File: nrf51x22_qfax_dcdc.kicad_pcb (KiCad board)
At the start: 2 copper layers, 14.8 x 16.4 mm, 46 parts, among them U1 nrf51822-qfax, X1 Crystal-4, X2 32.768kHz

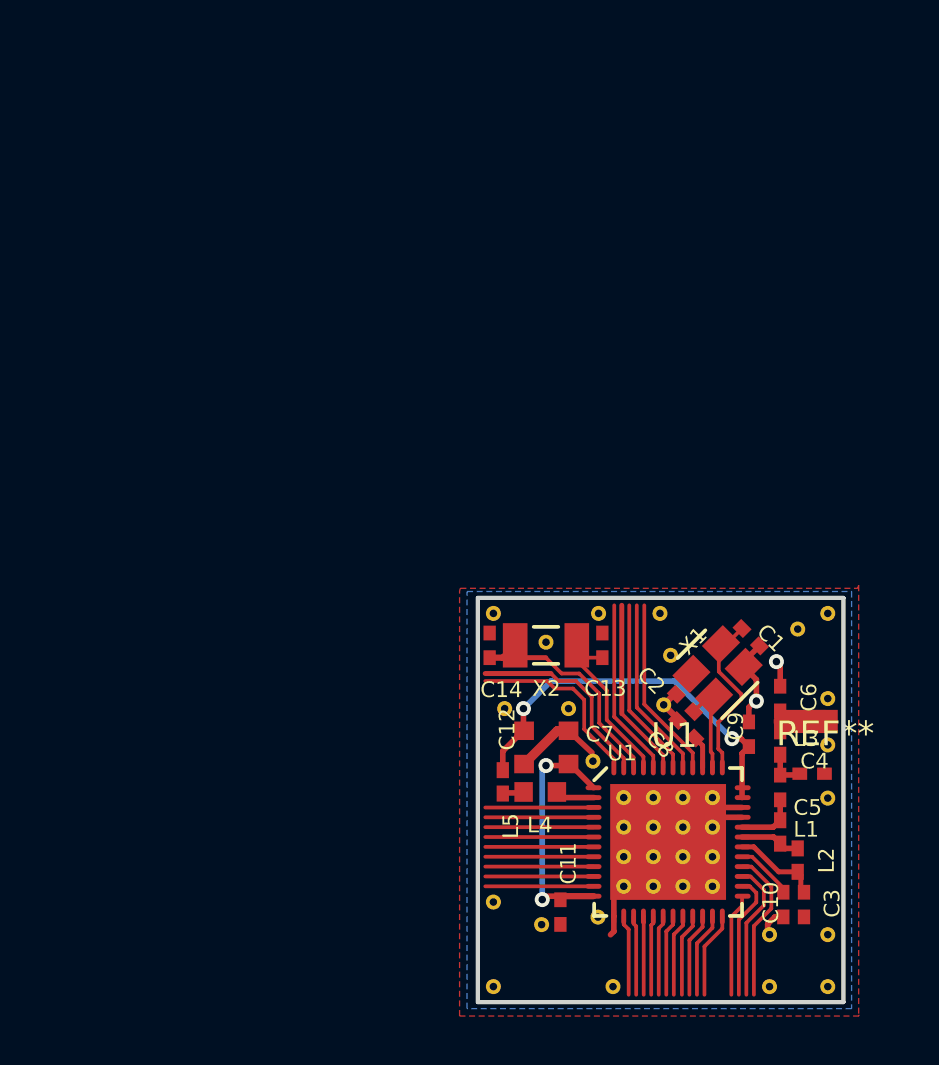
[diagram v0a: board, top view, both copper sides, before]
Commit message: WIP: Adding finished sch
Signed-off-by: Zamir SUN <sztsian@gmail.com>
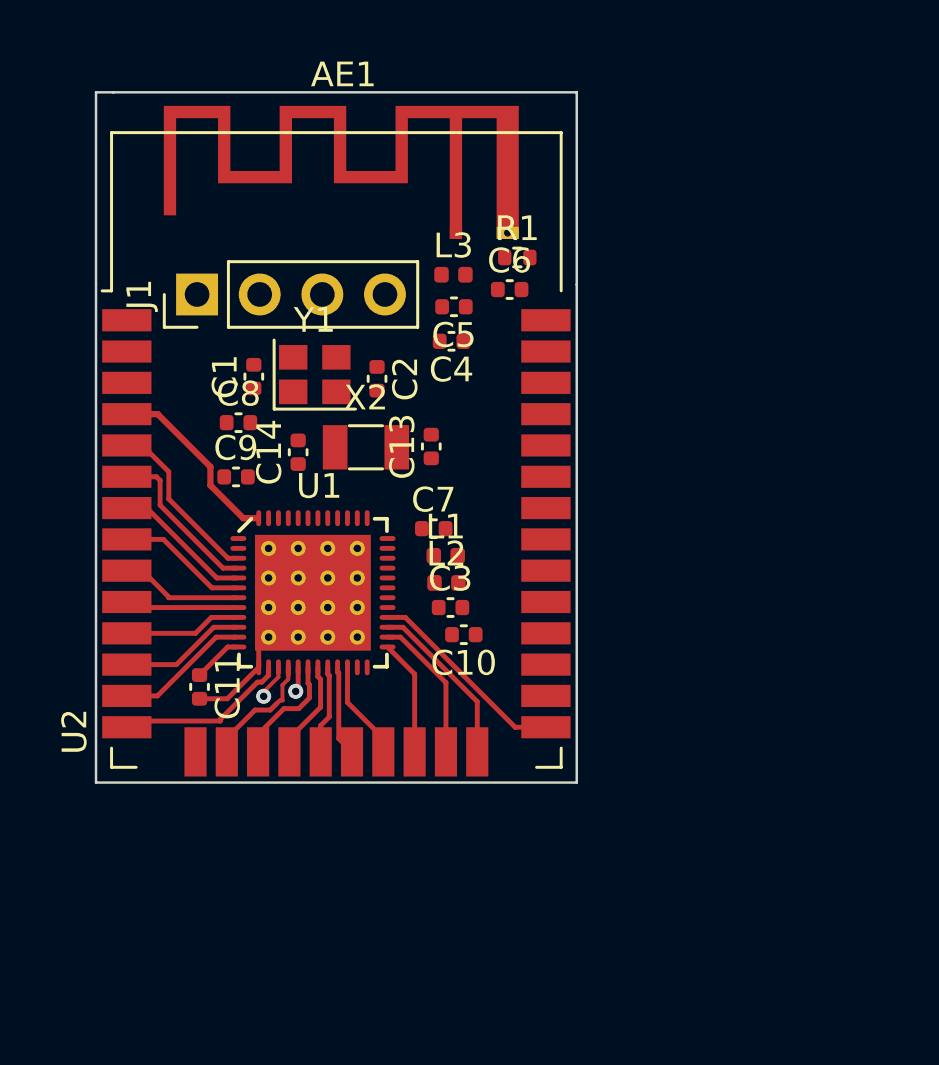
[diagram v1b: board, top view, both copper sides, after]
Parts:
- removed C12: 1.0uF, dcdc:CAPC1608X06L
- removed L4: 10uH, dcdc:INDC1608X06L
- removed L5: 15nH, dcdc:INDC1005X04L
- removed REF** (x23): VIA-0.6096, dcdc:VIA-0.6096
- removed REF**: antenna, dcdc:antenna
- removed X1: Crystal-4, dcdc:BT-XTAL_2520
- added AE1: Antenna_Chip, RF_Antenna:Texas_SWRA117D_2.4GHz_Left, F.Cu at (75.5, -110.2)
- added J1: SWD, Connector_PinHeader_2.54mm:PinHeader_1x04_P2.54mm_Vertical, F.Cu at (65.0, -107.7)
- added R1: 0R, Resistor_SMD:R_0402_1005Metric, F.Cu at (78.0, -109.2)
- added U2: nRF51822-WROOM-32, zsun-symbols:nRF51822-WROOM-32D, F.Cu at (70.7, -98.4)
- added Y1: 16M 3225, Crystal:Crystal_SMD_2520-4Pin_2.5x2.0mm, F.Cu at (69.8, -104.5)
- C1, C10, C11, C13, C14, C2, C3, C4, C5, C6, C8, C9: footprint dcdc:CAPC1005X04L -> Capacitor_SMD:C_0402_1005Metric
- C7: footprint dcdc:CAPC1608X06L -> Capacitor_SMD:C_0402_1005Metric
- L1, L2, L3: footprint dcdc:INDC1005X04L -> Inductor_SMD:L_0402_1005Metric
- X2: footprint dcdc:XTAL_3215 -> Crystal:Crystal_SMD_3215-2Pin_3.2x1.5mm
- moved C5 23.6 mm to (75.4, -107.2), turned to 180 degrees
- moved C9 23.3 mm to (66.6, -100.3), turned to 0 degrees
- moved L3 23.2 mm to (75.4, -108.5), turned to 0 degrees
- moved C4 22.8 mm to (75.3, -105.8), turned to 180 degrees
- moved C1 22.8 mm to (67.3, -104.4), turned to 90 degrees
- moved C8 22.0 mm to (66.7, -102.5), turned to 0 degrees
- moved C6 19.9 mm to (77.7, -107.9), turned to 0 degrees
- moved C3 18.7 mm to (75.3, -95.0), turned to 0 degrees
- moved L2 18.2 mm to (75.1, -96.0)
- moved C2 18.1 mm to (72.3, -104.3), turned to 270 degrees
- moved U1 17.6 mm to (69.7, -95.6)
- moved L1 17.6 mm to (75.1, -97.1)
- moved C11 17.3 mm to (65.1, -91.8)
- moved C10 17.0 mm to (75.8, -93.9), turned to 180 degrees
- moved C14 11.0 mm to (69.1, -101.3), turned to 90 degrees
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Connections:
- C11 pad 1: Net-(C11-Pad1) -> /AVDD
- C7 pad 1: Net-(C11-Pad1) -> /AVDD
- C9 pad 1: Net-(C12-Pad1) -> /AVDD
- U1 pad 1: Net-(C11-Pad1) -> /AVDD
- U1 pad 10: (no net) -> /P0.06
- U1 pad 11: (no net) -> /P0.07
- U1 pad 12: Net-(C11-Pad1) -> /AVDD
- U1 pad 14: (no net) -> /P0.08
- U1 pad 15: (no net) -> /P0.09
- U1 pad 16: (no net) -> /P0.10
- U1 pad 17: (no net) -> /P0.11
- U1 pad 18: (no net) -> /P0.12
- U1 pad 19: (no net) -> /P0.13
- U1 pad 2: Net-(L4-Pad2) -> (no net)
- U1 pad 20: (no net) -> /P0.14
- U1 pad 21: (no net) -> /P0.15
- U1 pad 22: (no net) -> /P0.16
- U1 pad 23: (no net) -> /SWDIO
- U1 pad 24: (no net) -> /SWCLK
- U1 pad 25: (no net) -> /P0.17
- U1 pad 26: (no net) -> /P0.18
- U1 pad 27: (no net) -> /P0.19
- U1 pad 28: (no net) -> /P0.20
- U1 pad 3: (no net) -> /P0.30
- U1 pad 35: Net-(C12-Pad1) -> /AVDD
- U1 pad 36: Net-(C12-Pad1) -> /AVDD
- U1 pad 4: (no net) -> /P0.00
- U1 pad 40: (no net) -> /P0.21
- U1 pad 41: (no net) -> /P0.22
- U1 pad 42: (no net) -> /P0.23
- U1 pad 43: (no net) -> /P0.24
- U1 pad 44: (no net) -> /P0.25
- U1 pad 47: (no net) -> /P0.28
- U1 pad 48: (no net) -> /P0.29
- U1 pad 5: (no net) -> /P0.01
- U1 pad 6: (no net) -> /P0.02
- U1 pad 7: (no net) -> /P0.03
- U1 pad 8: (no net) -> /P0.04
- U1 pad 9: (no net) -> /P0.05
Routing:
- net (no net): track 149.8 -> 0.00 mm
- net Net-(C12-Pad1): track 15.7 -> 0.00 mm, vias 2 -> 0
- net GND: track 19.3 -> 6.86 mm, vias 2 -> 0
- net Net-(C11-Pad1): track 11.2 -> 0.00 mm, vias 2 -> 0
- net Net-(C14-Pad2): track 9.89 -> 0.00 mm
- net /P0.20: track 0.00 -> 8.27 mm
- net /P0.29: track 0.00 -> 7.44 mm
- net /P0.08: track 0.00 -> 6.99 mm
- net /P0.30: track 0.00 -> 6.97 mm
- net /P0.19: track 0.00 -> 6.93 mm
- net Net-(C1-Pad1): track 6.86 -> 0.00 mm
- net /P0.00: track 0.00 -> 6.55 mm
- net Net-(C13-Pad2): track 6.04 -> 0.00 mm
- net /P0.18: track 0.00 -> 5.94 mm
- net /P0.01: track 0.00 -> 5.60 mm
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- removed copper zone on B.Cu, net GND
- removed copper zone on F.Cu, net GND
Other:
- board size 14.8 x 16.4 mm -> 19.5 x 28 mm
- board text removed: "C1"
- board text removed: "C10"
- board text removed: "C11"
- board text removed: "C12"
- board text removed: "C13"
- board text removed: "C14"
- board text removed: "C2"
- board text removed: "C3"
- board text removed: "C4"
- board text removed: "C5"
- board text removed: "C6"
- board text removed: "C7"
- board text removed: "C8"
- board text removed: "C9"
- board text removed: "L1"
- board text removed: "L2"
- board text removed: "L3"
- board text removed: "L4"
- board text removed: "L5"
- board text removed: "U1"
- board text removed: "X1"
- board text removed: "X2"

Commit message: WIP: finish basic pcb. There are errors in gerber
Signed-off-by: Ziqian SUN(Zamir) <zsun@redhat.com>
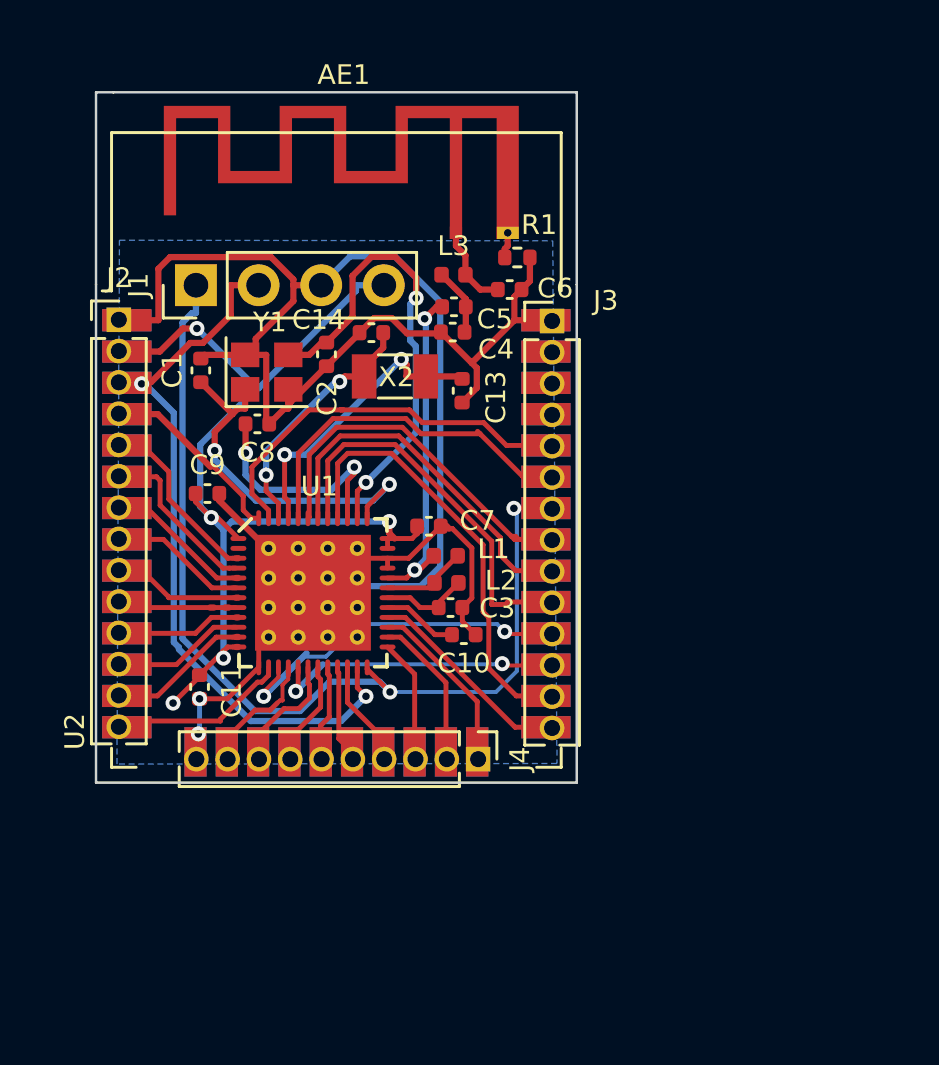
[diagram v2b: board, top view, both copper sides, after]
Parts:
- added J2: Conn_01x14_Male, Connector_PinHeader_1.27mm:PinHeader_1x14_P1.27mm_Vertical, F.Cu at (61.8, -106.7)
- added J3: Conn_01x14_Male, Connector_PinHeader_1.27mm:PinHeader_1x14_P1.27mm_Vertical, F.Cu at (79.4, -106.6)
- added J4: Conn_01x10_Male, Connector_PinHeader_1.27mm:PinHeader_1x10_P1.27mm_Vertical, F.Cu at (76.4, -88.8)
- added U3: nRF51822-WROOM-32, zsun-symbols:nRF51822-WROOM-32D, B.Cu at (70.7, -98.4)
- moved C14 5.69 mm to (72.1, -106.2), turned to 0 degrees
- moved X2 3.11 mm to (73.0, -104.4)
- moved C13 2.58 mm to (75.8, -103.8)
- moved C2 2.28 mm to (70.2, -105.3)
- moved C1 2.16 mm to (65.2, -104.6)
- moved Y1 1.95 mm to (67.8, -104.5)
- moved C9 1.34 mm to (65.4, -99.6)
- moved C8 0.77 mm to (67.4, -102.5), turned to 180 degrees
- moved C4 0.38 mm to (75.4, -106.2)
- moved J1 0.38 mm to (65.0, -108.1)
- moved C7 0.22 mm to (74.4, -98.3)
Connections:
- J1 pad 4: /AVDD -> /VCC_nRF
- U1 pad 2: (no net) -> Net-(U1-Pad2)
- U2 pad 32: (no net) -> /SWCLK
- U2 pad 35: (no net) -> Net-(U2-Pad35)
- U2 pad 36: (no net) -> Net-(U2-Pad36)
- U2 pad 37: (no net) -> Net-(U2-Pad37)
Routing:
- net GND: track 6.86 -> 98.8 mm, vias 0 -> 2
- net /AVDD: track 1.95 -> 42.5 mm, vias 0 -> 5
- net /SWCLK: track 0.00 -> 39.8 mm, vias 0 -> 2
- net /SWDIO: track 0.00 -> 30.2 mm, vias 0 -> 2
- net Net-(C2-Pad1): track 0.00 -> 19.1 mm, vias 0 -> 2
- net /P0.21: track 0.00 -> 17.7 mm
- net /P0.22: track 0.00 -> 16.2 mm
- net /P0.09: track 1.42 -> 17.6 mm, vias 1 -> 2
- net /P0.24: track 0.00 -> 16.0 mm
- net /P0.28: track 0.00 -> 15.9 mm
- net Net-(C1-Pad1): track 0.00 -> 15.2 mm, vias 0 -> 2
- net /P0.23: track 0.00 -> 14.7 mm
- net /P0.25: track 0.00 -> 14.4 mm
- net Net-(C5-Pad2): track 0.00 -> 13.7 mm, vias 0 -> 2
- net Net-(C13-Pad2): track 0.00 -> 12.0 mm, vias 0 -> 2
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- added copper zone on B.Cu, net GND
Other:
- net class Default: clearance 0.1524 -> 0.1; trace_width 0.254 -> 0.1
- net class Net-(C6-Pad1): clearance 0.1524 -> 0.1
- rule trace_clearance: 0.1524 -> 0.1
- rule trace_min: 0.152 -> 0.1
- board text added: "3v3 GND DIO CLK"
- board text added: "GND P10 P12 P13 P14 P15 P16 P17 P18 P19"
- board text added: "GND VDD DIO P20 P30 P00 P01 P02 P03 P04 P05 P06 P07"
- board text added: "GND X X X P28 P25 CLK P24 P23 P22 P09 P11 P21"
- board text added: "P08"
- board text added: "P20"
- board text added: "nRF51822 WROOM"
